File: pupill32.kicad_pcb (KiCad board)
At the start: 2 copper layers, 52.1 x 27.9 mm, 54 parts, among them J1 HeaderR, J2 HeaderL, J3 USB_PINS, J4 SWD_HEADER, SW1 RST_BTN, SW2 BOOT_BTN, U1 SRV05-4, U2 PY32F030F18P6, U3 CH340N, U4 AMS1117-3.3, Y1 32.768 kHz, Y2 12M

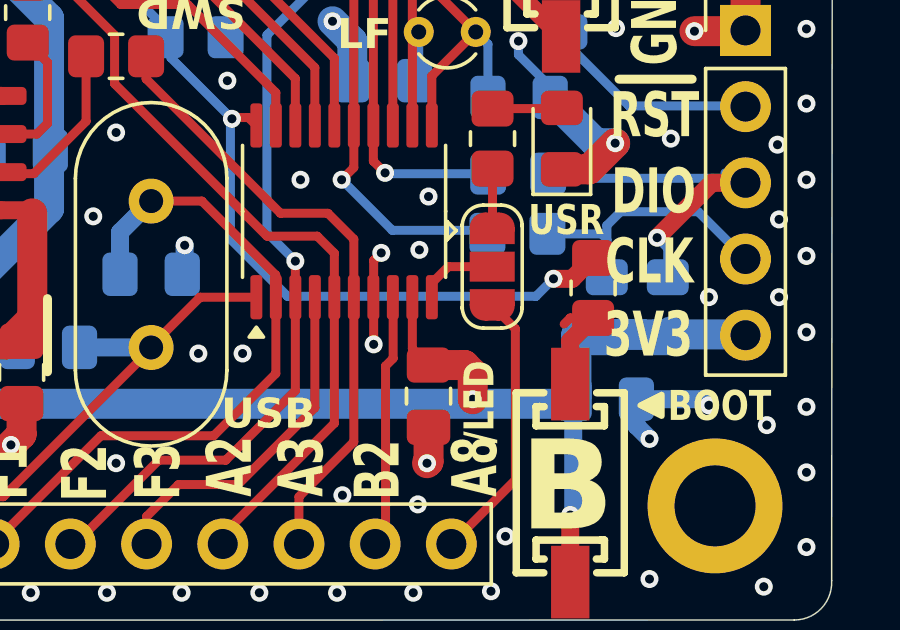
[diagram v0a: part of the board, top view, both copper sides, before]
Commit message: minor tuning
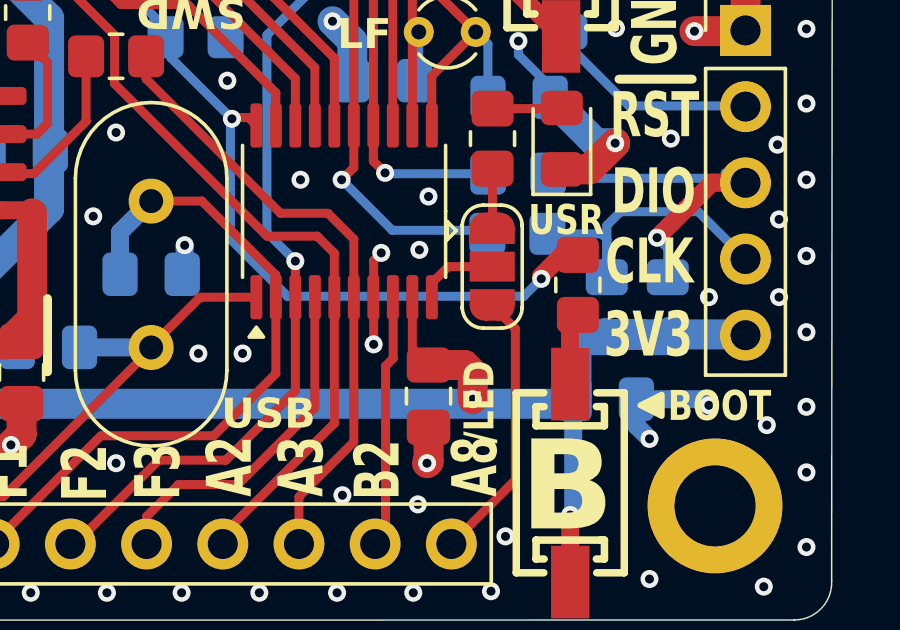
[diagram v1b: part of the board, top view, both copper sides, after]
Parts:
- moved R8 0.52 mm to (133.8, 79.0)
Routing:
- net Net-(R8-Pad1): track 3.57 -> 2.41 mm
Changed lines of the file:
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@@
 	(footprint "Resistor_SMD:R_0805_2012Metric_Pad1.20x1.40mm_HandSolder"
 		(layer "F.Cu")
-		(at 134.2644 79.0956 90)
+		(at 133.7564 78.994 90)
 		(descr "Resistor SMD 0805 (2012 Metric), square (rectangular) end terminal, IPC_7351 nominal with elongated pad for handsoldering. (Body size source: IPC-SM-782 page 72, https://www.pcb-3d.com/wordpress/wp-content/uploads/ipc-sm-782a_amendment_1_and_2.pdf), generated with kicad-footprint-generator")
 		(tags "resistor handsolder")
@@
 	)
 	(segment
-		(start 132.9436 78.7908)
-		(end 133.5692 78.7908)
+		(start 132.5372 78.6892)
+		(end 133.2324 77.994)
+		(width 0.6)
+		(layer "F.Cu")
+		(net 36)
+	)
+	(segment
+		(start 132.5372 78.7908)
+		(end 132.5372 78.6892)
+		(width 0.6)
+		(layer "F.Cu")
+		(net 36)
+	)
+	(segment
+		(start 133.2324 77.994)
+		(end 133.7564 77.994)
 		(width 0.6)
 		(layer "F.Cu")
@@
 		(net 36)
 	)
-	(segment
-		(start 133.5692 78.7908)
-		(end 134.2644 78.0956)
-		(width 0.6)
-		(layer "F.Cu")
-		(net 36)
-	)
 	(via
 		(at 122.2248 73.4568)
@@
 	)
 	(via
-		(at 132.9436 78.7908)
+		(at 132.5372 78.7908)
 		(size 0.6)
 		(drill 0.3)
@@
 	)
 	(segment
-		(start 122.174 73.5076)
-		(end 122.2248 73.4568)
-		(width 0.3)
-		(layer "B.Cu")
-		(net 36)
-	)
-	(segment
-		(start 122.174 77.47)
-		(end 122.174 73.5076)
-		(width 0.3)
-		(layer "B.Cu")
-		(net 36)
-	)
-	(segment
 		(start 108.4072 66.802)
 		(end 116.3828 66.802)
@@
 	)
 	(segment
-		(start 124.079 79.375)
-		(end 122.174 77.47)
+		(start 122.174 73.5076)
+		(end 122.2248 73.4568)
 		(width 0.3)
 		(layer "B.Cu")
@@
 	)
 	(segment
+		(start 132.5372 78.7908)
+		(end 131.953 79.375)
+		(width 0.3)
+		(layer "B.Cu")
+		(net 36)
+	)
+	(segment
 		(start 120.1928 70.612)
 		(end 120.1928 71.4248)
@@
 	)
 	(segment
-		(start 132.3594 79.375)
-		(end 124.079 79.375)
+		(start 122.174 77.47)
+		(end 122.174 73.5076)
 		(width 0.3)
 		(layer "B.Cu")
@@
 	)
 	(segment
-		(start 132.9436 78.7908)
-		(end 132.3594 79.375)
+		(start 124.079 79.375)
+		(end 122.174 77.47)
 		(width 0.3)
 		(layer "B.Cu")
@@
 	)
 	(segment
+		(start 131.953 79.375)
+		(end 124.079 79.375)
+		(width 0.3)
+		(layer "B.Cu")
+		(net 36)
+	)
+	(segment
 		(start 106.68 65.0748)
 		(end 108.4072 66.802)
@@
 	)
 	(segment
-		(start 133.5024 80.0956)
-		(end 134.2644 80.0956)
-		(width 0.3)
-		(layer "F.Cu")
-		(net 38)
-	)
-	(segment
-		(start 133.2992 80.2988)
-		(end 133.5024 80.0956)
-		(width 0.3)
-		(layer "F.Cu")
-		(net 38)
-	)
-	(segment
-		(start 133.5024 80.8576)
-		(end 134.2644 80.0956)
+		(start 133.5024 80.248)
+		(end 133.7564 79.994)
 		(width 0.6)
 		(layer "F.Cu")
@@
 	(segment
 		(start 133.5024 82.3)
-		(end 133.5024 80.8576)
+		(end 133.5024 80.248)
 		(width 0.6)
 		(layer "F.Cu")
